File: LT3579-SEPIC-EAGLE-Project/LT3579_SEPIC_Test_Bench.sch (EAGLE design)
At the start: 121 parts

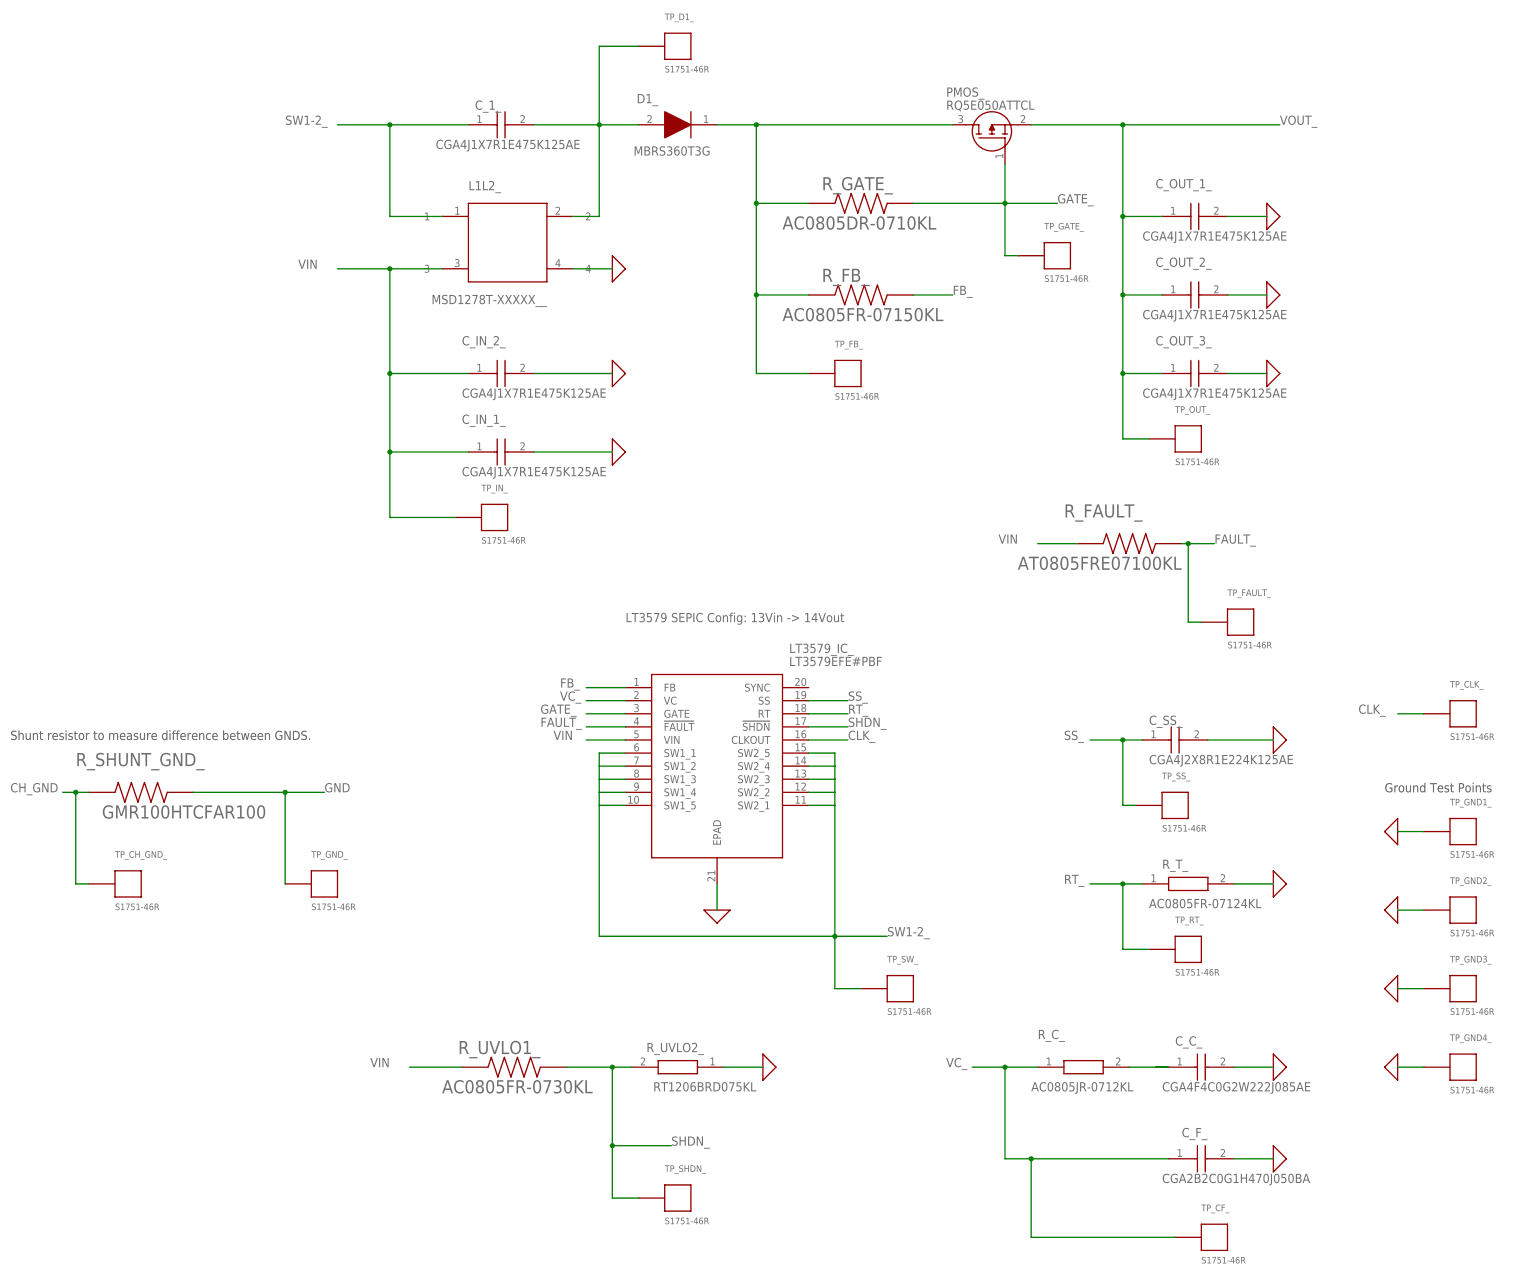
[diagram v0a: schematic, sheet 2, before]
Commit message: Modfied Schematic files eagle
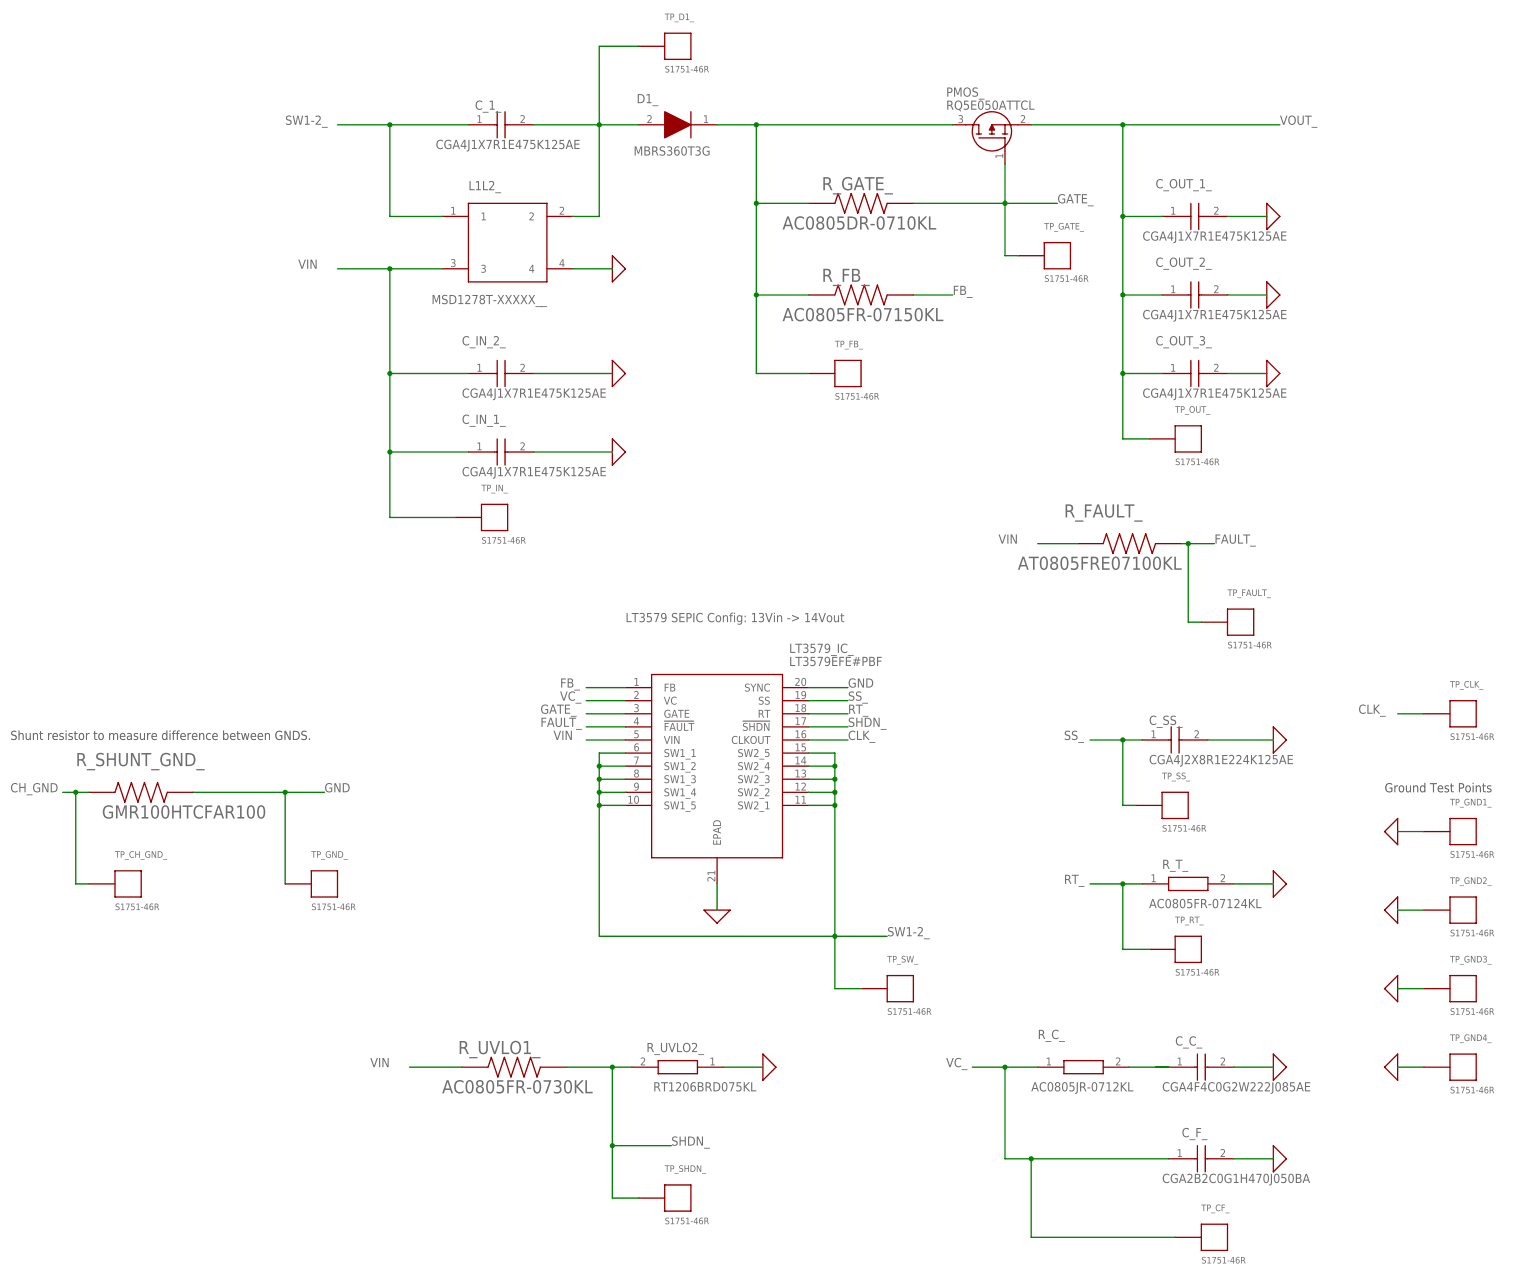
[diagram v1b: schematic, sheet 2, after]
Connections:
- net GND: now also LT3579_IC_.SYNC, LT3579_IC_1.SYNC, LT3579_IC_2.SYNC
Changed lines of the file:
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@@
 <setting verticaltext="up"/>
 </settings>
-<grid distance="0.1" unitdist="inch" unit="inch" style="lines" multiple="1" display="yes" altdistance="0.01" altunitdist="inch" altunit="inch"/>
+<grid distance="0.1" unitdist="inch" unit="inch" style="lines" multiple="1" display="no" altdistance="0.01" altunitdist="inch" altunit="inch"/>
 <layers>
 <layer number="1" name="Top" color="4" fill="1" visible="no" active="no"/>
@@
 <wire x1="22.86" y1="-45.72" x2="27.94" y2="-45.72" width="0.1524" layer="91"/>
 <junction x="22.86" y="-35.56"/>
+<junction x="-22.86" y="-2.54"/>
+<junction x="-22.86" y="-5.08"/>
+<junction x="-22.86" y="-7.62"/>
+<junction x="-22.86" y="-10.16"/>
+<junction x="22.86" y="-10.16"/>
+<junction x="22.86" y="-7.62"/>
+<junction x="22.86" y="-5.08"/>
+<junction x="22.86" y="-2.54"/>
 </segment>
 <segment>
@@
 <wire x1="-83.82" y1="-25.4" x2="-83.82" y2="-7.62" width="0.1524" layer="91"/>
 <junction x="-83.82" y="-7.62"/>
+</segment>
+<segment>
+<pinref part="LT3579_IC_" gate="G$1" pin="SYNC"/>
+<wire x1="17.78" y1="12.7" x2="25.4" y2="12.7" width="0.1524" layer="91"/>
+<label x="25.4" y="12.7" size="1.778" layer="95"/>
 </segment>
 </net>
@@
 <wire x1="22.86" y1="-43.18" x2="27.94" y2="-43.18" width="0.1524" layer="91"/>
 <junction x="22.86" y="-33.02"/>
+<junction x="22.86" y="0"/>
+<junction x="22.86" y="-2.54"/>
+<junction x="22.86" y="-5.08"/>
+<junction x="22.86" y="-7.62"/>
+<junction x="-22.86" y="-7.62"/>
+<junction x="-22.86" y="-5.08"/>
+<junction x="-22.86" y="-2.54"/>
+<junction x="-22.86" y="0"/>
 </segment>
 <segment>
@@
 <wire x1="-83.82" y1="-22.86" x2="-83.82" y2="-5.08" width="0.1524" layer="91"/>
 <junction x="-83.82" y="-5.08"/>
+</segment>
+<segment>
+<pinref part="LT3579_IC_1" gate="G$1" pin="SYNC"/>
+<wire x1="17.78" y1="15.24" x2="25.4" y2="15.24" width="0.1524" layer="91"/>
+<label x="25.4" y="15.24" size="1.778" layer="95"/>
 </segment>
 </net>
@@
 <wire x1="22.86" y1="-43.18" x2="27.94" y2="-43.18" width="0.1524" layer="91"/>
 <junction x="22.86" y="-33.02"/>
+<junction x="-22.86" y="0"/>
+<junction x="-22.86" y="-2.54"/>
+<junction x="-22.86" y="-5.08"/>
+<junction x="-22.86" y="-7.62"/>
+<junction x="22.86" y="-7.62"/>
+<junction x="22.86" y="-5.08"/>
+<junction x="22.86" y="-2.54"/>
+<junction x="22.86" y="0"/>
 </segment>
 <segment>
@@
 <junction x="-83.82" y="-5.08"/>
 </segment>
-</net>
+<segment>
+<pinref part="LT3579_IC_2" gate="G$1" pin="SYNC"/>
+<wire x1="17.78" y1="15.24" x2="25.4" y2="15.24" width="0.1524" layer="91"/>
+<label x="25.4" y="15.24" size="1.778" layer="95"/>
+</segment>
+</net>
